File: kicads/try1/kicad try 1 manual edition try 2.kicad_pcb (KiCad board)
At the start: 2 copper layers, 35 parts, among them P2 GND, P3 CONN_01X08, P4 A2 A3 A4 A5 A6, P5 Mutual, P6 CONN_01X08, SW1 SW_PUSH, SW2 SW_PUSH, SW3 SW_PUSH, SW4 SW_PUSH, U2 CD74HCT4067, U3 CD74HCT4067

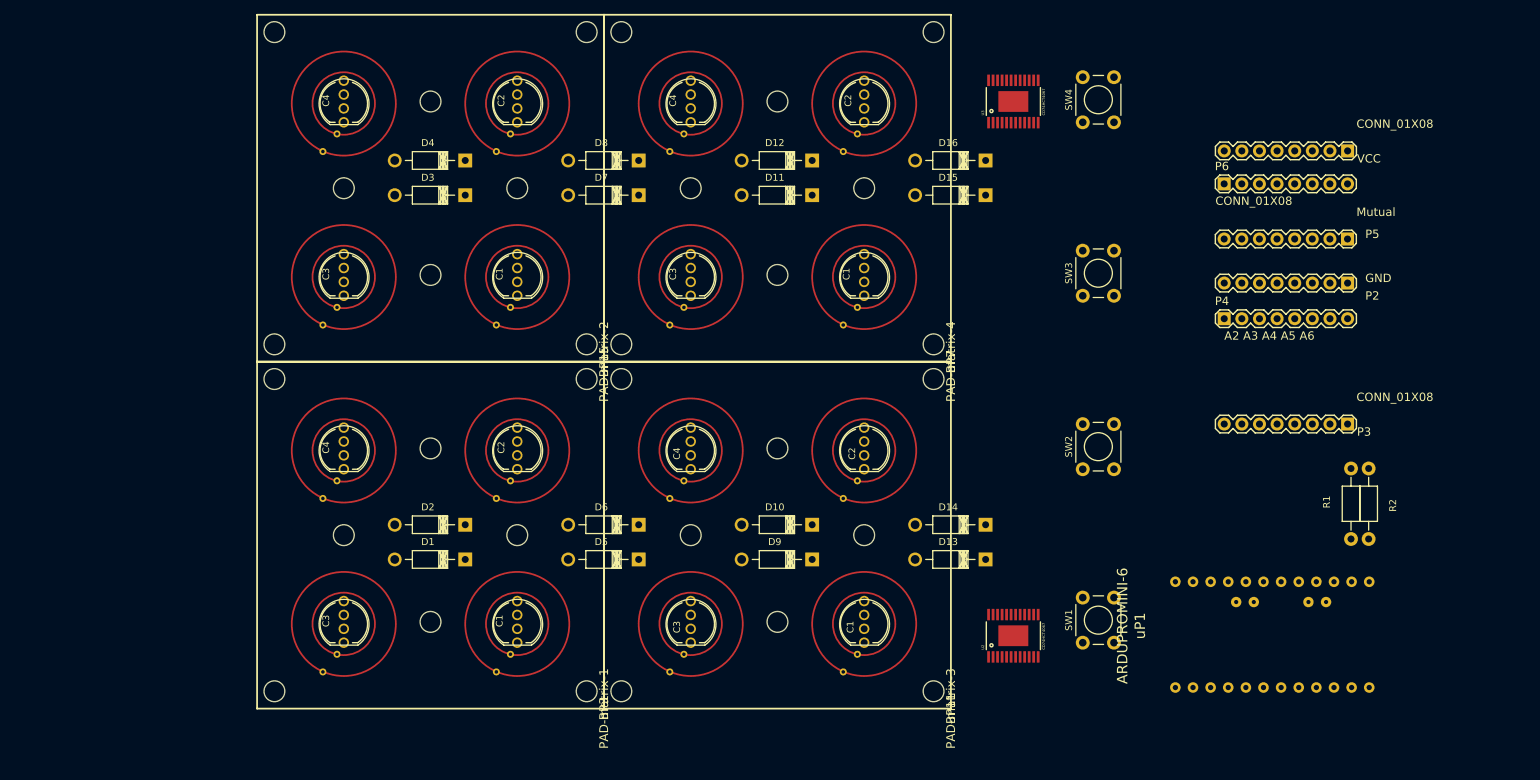
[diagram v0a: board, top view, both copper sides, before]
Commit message: forward with the pcb design
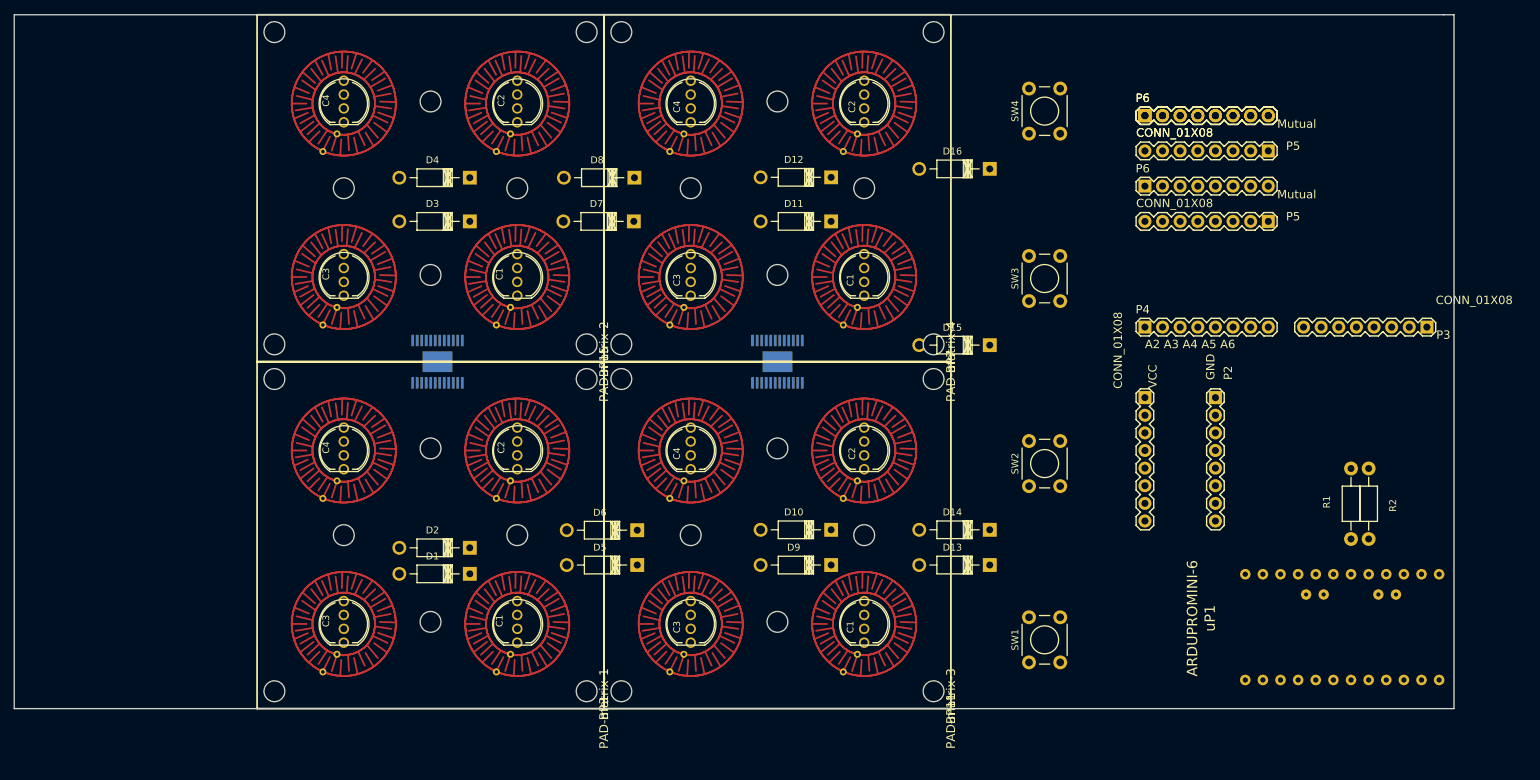
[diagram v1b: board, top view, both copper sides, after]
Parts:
- added P5: Mutual, SparkFun-Connectors:1X08, F.Cu at (205.7, 71.1)
- added P6 (x2): CONN_01X08, SparkFun-Connectors:1X08, F.Cu at (188.0, 66.0)
- U2, U3: moved to B.Cu
- moved U2 91.9 mm to (86.0, 101.5)
- moved U3 50.6 mm to (135.0, 101.5)
- moved VCC 46.0 mm to (188.0, 106.7), turned to 270 degrees
- moved P2 25.2 mm to (198.1, 106.7), turned to 270 degrees
- moved D15 21.6 mm to (165.6, 99.1)
- moved P3 18.1 mm to (228.6, 96.5)
- moved P5 11.7 mm to (205.7, 81.3)
- moved P4 11.5 mm to (188.0, 96.5)
- moved P6 11.4 mm to (188.0, 76.2)
- moved uP1 10.1 mm to (196.1, 149.9)
- moved SW1 8.25 mm to (171.3, 144.8)
- moved SW2 8.12 mm to (171.3, 119.4)
- moved SW4 7.92 mm to (171.3, 68.6)
- moved SW3 7.78 mm to (171.3, 92.8)
- moved D11 4.66 mm to (142.7, 81.3)
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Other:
- board outline added: 207.5 x 100 mm
- net class Default: clearance 0.4 -> 0.2032; trace_width 0.4 -> 0.2032; via_dia 0.6 -> 0.7493; via_drill 0.4 -> 0.50038
- rule trace_clearance: 0.4 -> 0.2032
